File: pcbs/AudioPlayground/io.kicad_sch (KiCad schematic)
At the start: 22 parts, among them J1 Conn_01x07_Socket, J2 Conn_Battery, J5 Conn_01x12_Pin, J7 Conn_01x16_Pin, J9 Conn_01x07_Socket, U7 DMM-4326-T-R, U8 DMM-4326-T-R

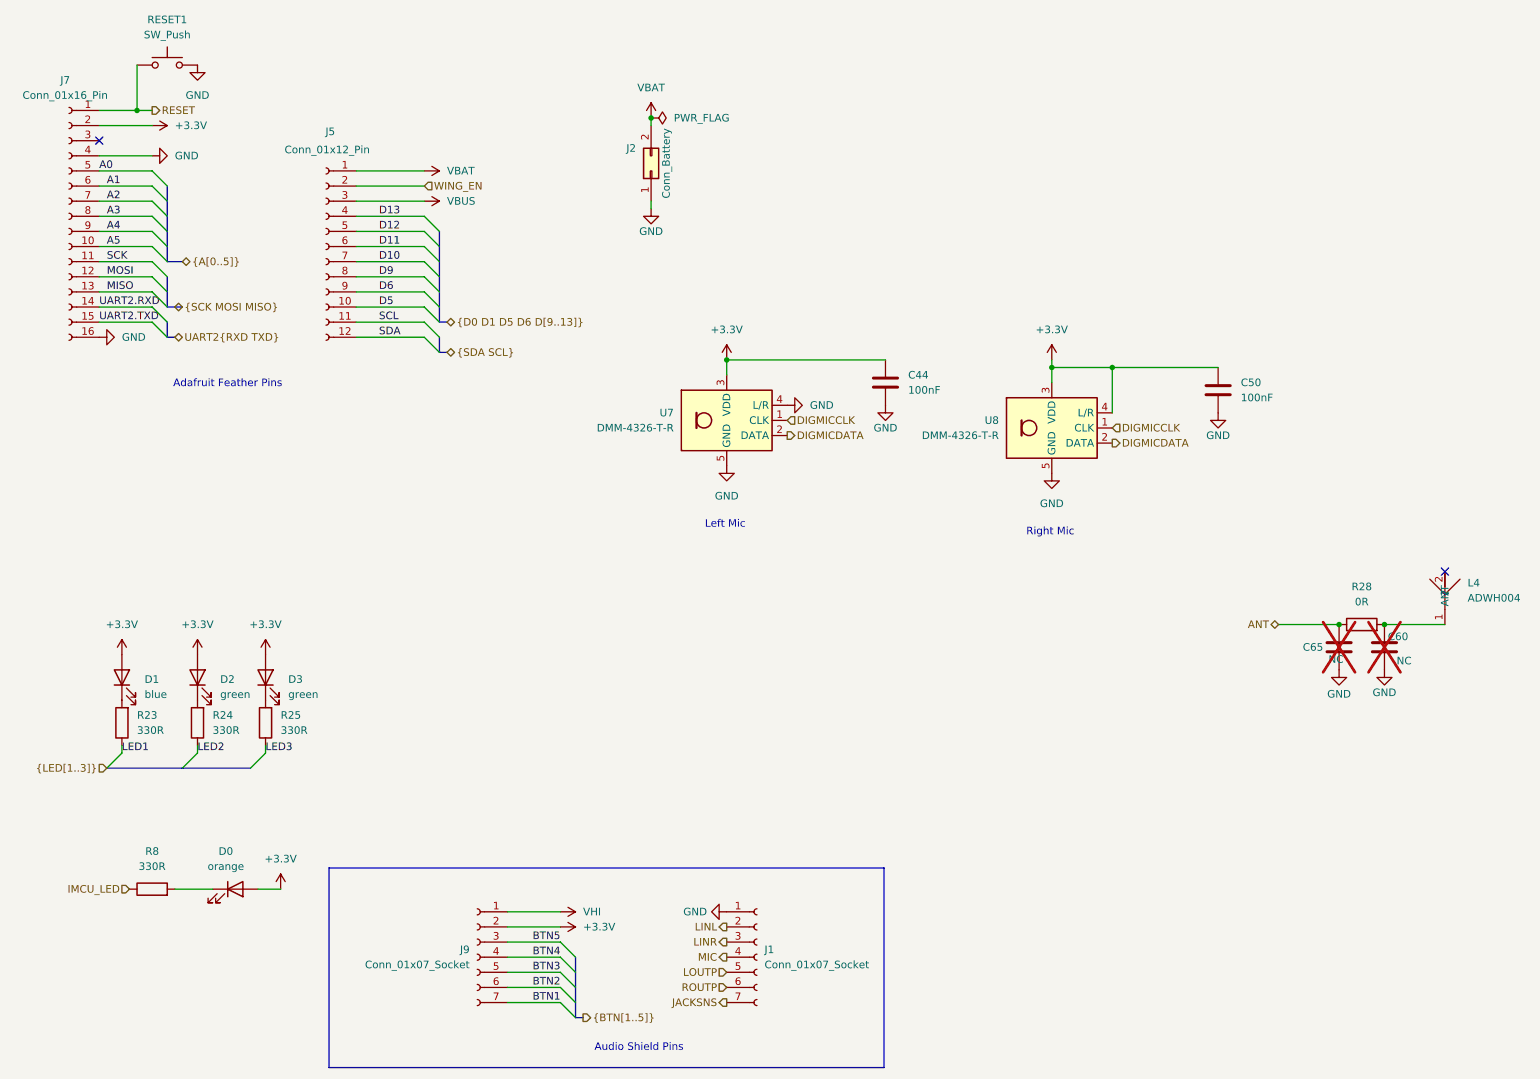
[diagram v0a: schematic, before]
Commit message: Update MICs
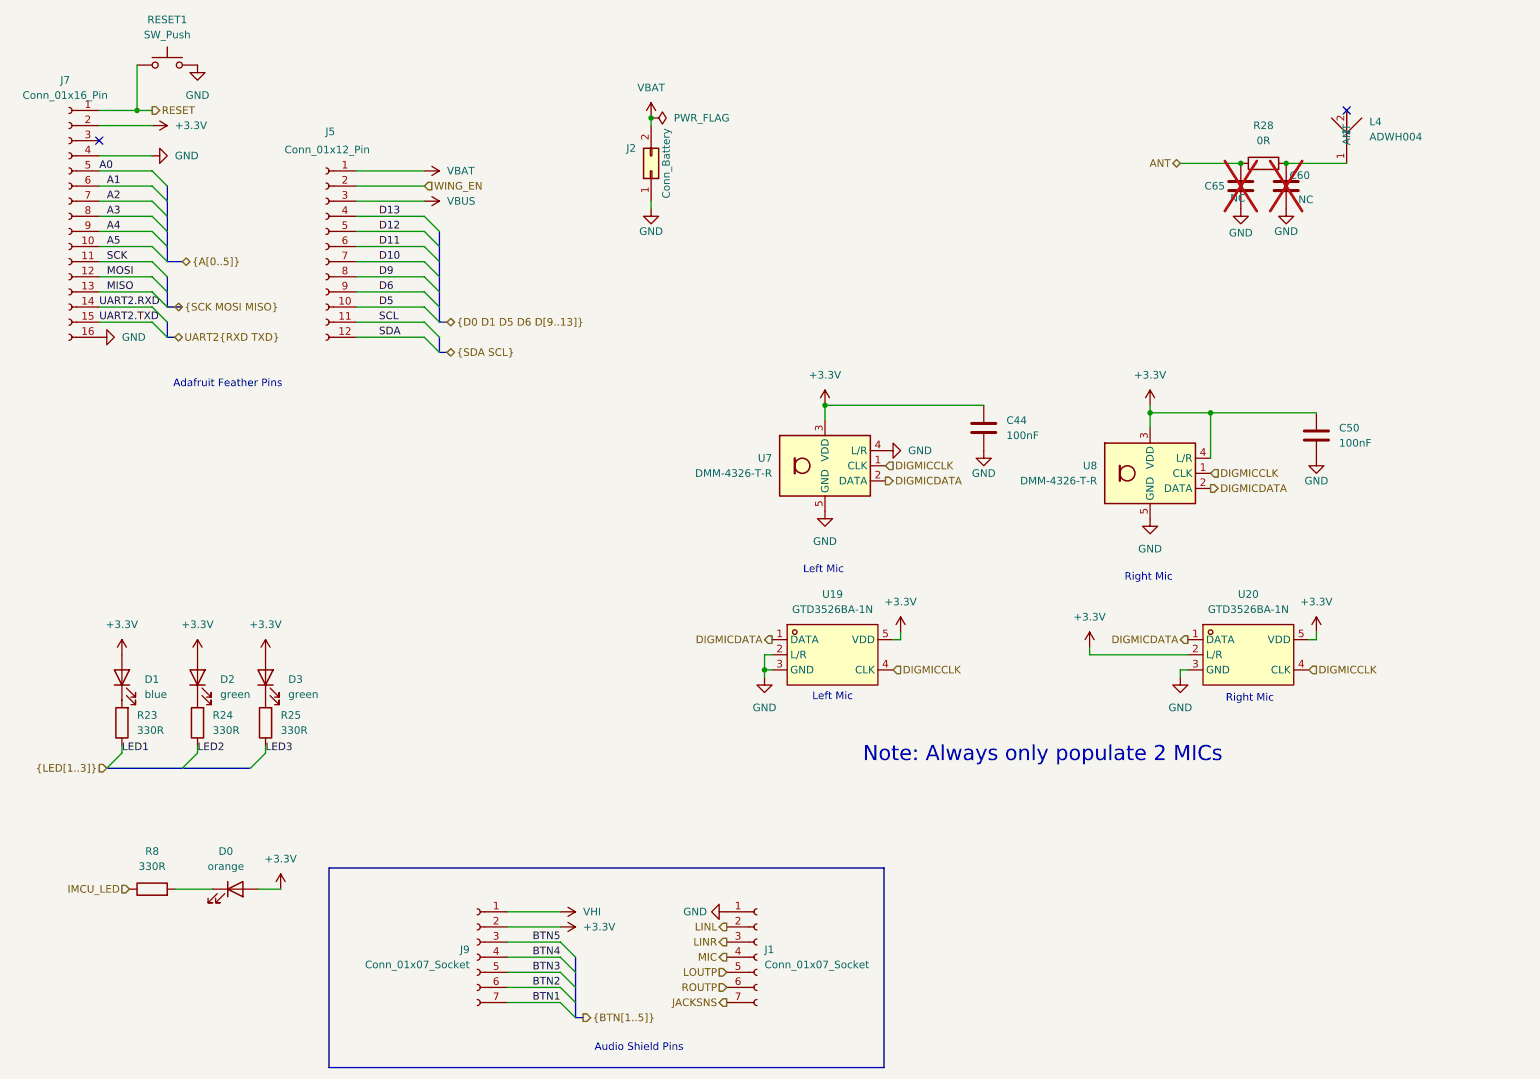
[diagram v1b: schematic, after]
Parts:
- added U19, U20: GTD3526BA-1N, GTD3526BA-1N:GTD3526BA-1N, symbol GTD3526BA-1N:GTD3526BA-1N
- U7, U8: LCSC (none) -> C47148415
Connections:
- net +3.3V: now also U19.5 (VDD), U20.2 (L/R), U20.5 (VDD)
- net DIGMICCLK: now also U19.4 (CLK), U20.4 (CLK)
- net DIGMICDATA: now also U19.1 (DATA), U20.1 (DATA)
- net GND: now also U19.2 (L/R), U19.3 (GND), U20.3 (GND)
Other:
- note added: "Note: Always only populate 2 MICs"
- moved on the sheet: C44, C50, C60, C65, L4, R28, U7, U8
